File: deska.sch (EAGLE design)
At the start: 14 parts, among them T1 TIP122, T2 TIP122, T3 TIP122, X2 NAPAJENI

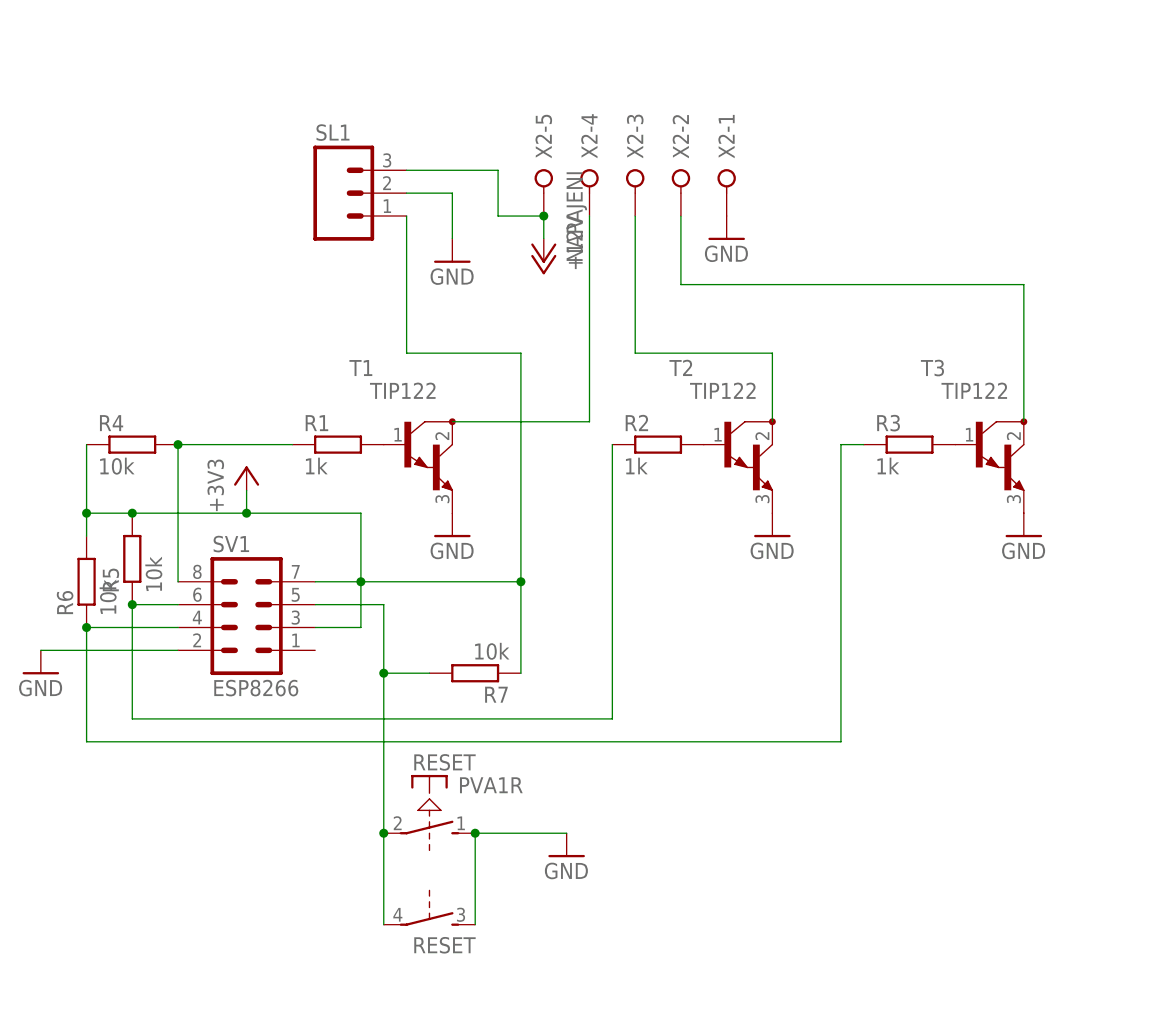
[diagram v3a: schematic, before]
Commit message: upravy desky
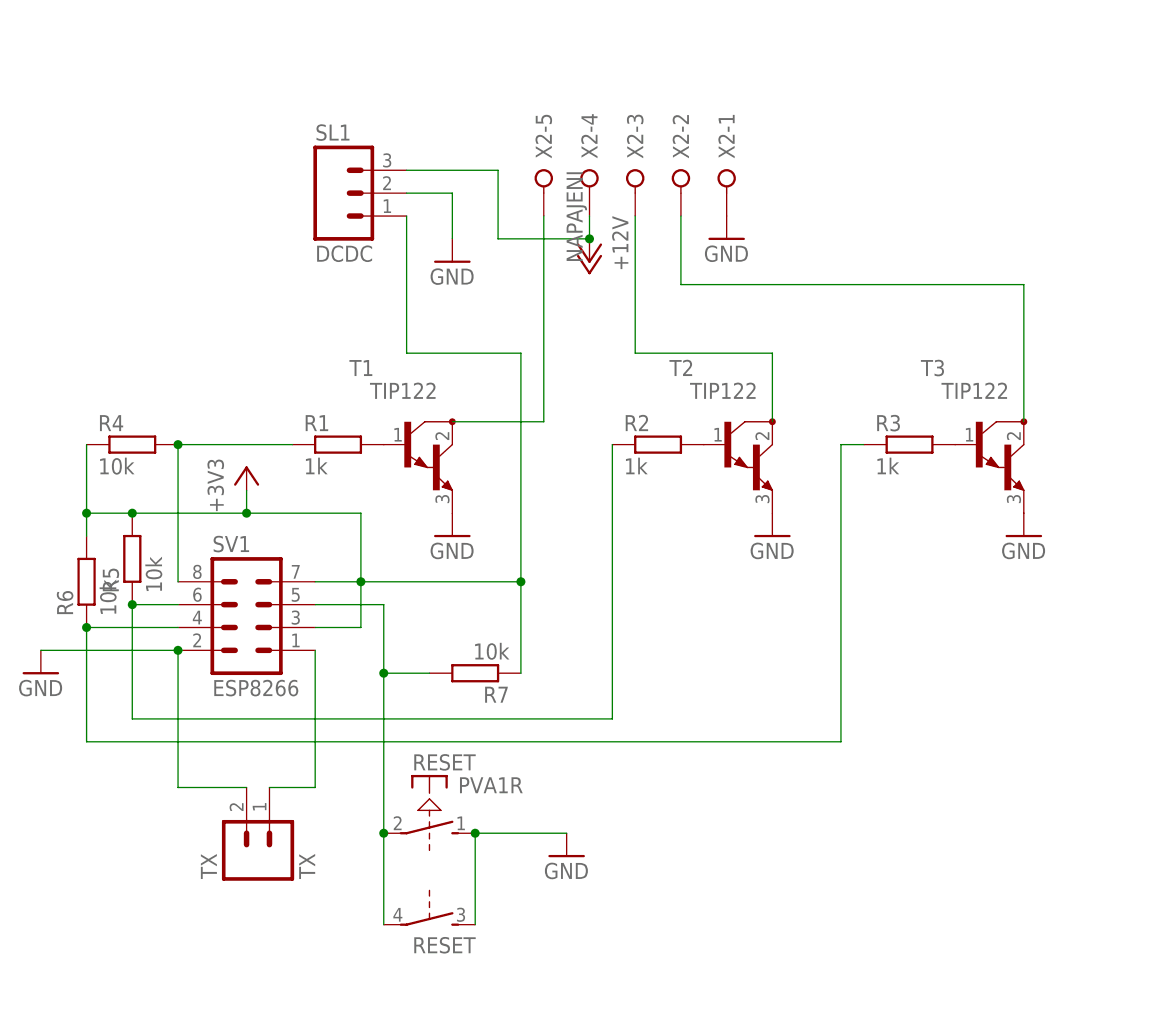
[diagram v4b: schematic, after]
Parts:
- added TX: TX, con-amp-quick:M02
- SL1: value (none) -> DCDC
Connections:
- new net N$9: SV1.1, TX.1
- net +12V: now also X2-4.KL; no longer X2-5.KL
- net GND: now also TX.2
- net N$1: now also X2-5.KL; no longer X2-4.KL
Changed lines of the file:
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@@
 <part name="GND7" library="supply1" deviceset="GND" device=""/>
 <part name="+3V1" library="supply1" library_urn="urn:adsk.eagle:library:371" deviceset="+3V3" device=""/>
-<part name="SL1" library="con-amp-quick" library_urn="urn:adsk.eagle:library:125" deviceset="M03" device="" package3d_urn="urn:adsk.eagle:package:5957/1"/>
+<part name="SL1" library="con-amp-quick" library_urn="urn:adsk.eagle:library:125" deviceset="M03" device="" package3d_urn="urn:adsk.eagle:package:5957/1" value="DCDC"/>
 <part name="GND5" library="supply1" deviceset="GND" device=""/>
+<part name="TX" library="con-amp-quick" library_urn="urn:adsk.eagle:library:125" deviceset="M02" device="" package3d_urn="urn:adsk.eagle:package:5956/1" value="TX"/>
 </parts>
 <sheets>
@@
 <instance part="GND2" gate="1" x="58.42" y="55.88"/>
 <instance part="GND3" gate="1" x="86.36" y="55.88"/>
-<instance part="P+1" gate="1" x="33.02" y="86.36" rot="R180"/>
+<instance part="P+1" gate="1" x="38.1" y="86.36" rot="R180"/>
 <instance part="R1" gate="G$1" x="10.16" y="66.04"/>
 <instance part="R2" gate="G$1" x="45.72" y="66.04"/>
@@
 <instance part="SL1" gate="G$1" x="10.16" y="93.98"/>
 <instance part="GND5" gate="1" x="22.86" y="86.36"/>
+<instance part="TX" gate="G$1" x="2.54" y="20.32" rot="R90"/>
 </instances>
 <busses>
@@
 <wire x1="-22.86" y1="43.18" x2="-7.62" y2="43.18" width="0.1524" layer="91"/>
 <pinref part="SV1" gate="G$1" pin="2"/>
+<pinref part="TX" gate="G$1" pin="2"/>
+<wire x1="0" y1="27.94" x2="-7.62" y2="27.94" width="0.1524" layer="91"/>
+<wire x1="-7.62" y1="27.94" x2="-7.62" y2="43.18" width="0.1524" layer="91"/>
+<junction x="-7.62" y="43.18"/>
 </segment>
 <segment>
@@
 </segment>
 </net>
-<net name="+12V" class="0">
-<segment>
-<pinref part="P+1" gate="1" pin="+12V"/>
-<wire x1="33.02" y1="88.9" x2="33.02" y2="91.44" width="0.1524" layer="91"/>
+<net name="N$1" class="0">
+<segment>
+<pinref part="T1" gate="G$1" pin="C"/>
+<wire x1="22.86" y1="68.58" x2="33.02" y2="68.58" width="0.1524" layer="91"/>
 <pinref part="X2" gate="-5" pin="KL"/>
-<pinref part="SL1" gate="G$1" pin="3"/>
-<wire x1="17.78" y1="96.52" x2="27.94" y2="96.52" width="0.1524" layer="91"/>
-<wire x1="27.94" y1="96.52" x2="27.94" y2="91.44" width="0.1524" layer="91"/>
-<wire x1="27.94" y1="91.44" x2="33.02" y2="91.44" width="0.1524" layer="91"/>
-<junction x="33.02" y="91.44"/>
-</segment>
-</net>
-<net name="N$1" class="0">
-<segment>
-<pinref part="T1" gate="G$1" pin="C"/>
-<wire x1="22.86" y1="68.58" x2="38.1" y2="68.58" width="0.1524" layer="91"/>
-<wire x1="38.1" y1="68.58" x2="38.1" y2="91.44" width="0.1524" layer="91"/>
-<pinref part="X2" gate="-4" pin="KL"/>
+<wire x1="33.02" y1="91.44" x2="33.02" y2="68.58" width="0.1524" layer="91"/>
 </segment>
 </net>
@@
 </segment>
 </net>
+<net name="N$9" class="0">
+<segment>
+<pinref part="SV1" gate="G$1" pin="1"/>
+<wire x1="7.62" y1="43.18" x2="7.62" y2="27.94" width="0.1524" layer="91"/>
+<pinref part="TX" gate="G$1" pin="1"/>
+<wire x1="7.62" y1="27.94" x2="2.54" y2="27.94" width="0.1524" layer="91"/>
+</segment>
+</net>
+<net name="+12V" class="0">
+<segment>
+<pinref part="X2" gate="-4" pin="KL"/>
+<pinref part="P+1" gate="1" pin="+12V"/>
+<wire x1="38.1" y1="88.9" x2="38.1" y2="91.44" width="0.1524" layer="91"/>
+<pinref part="SL1" gate="G$1" pin="3"/>
+<wire x1="17.78" y1="96.52" x2="27.94" y2="96.52" width="0.1524" layer="91"/>
+<wire x1="27.94" y1="96.52" x2="27.94" y2="88.9" width="0.1524" layer="91"/>
+<wire x1="27.94" y1="88.9" x2="38.1" y2="88.9" width="0.1524" layer="91"/>
+<junction x="38.1" y="88.9"/>
+</segment>
+</net>

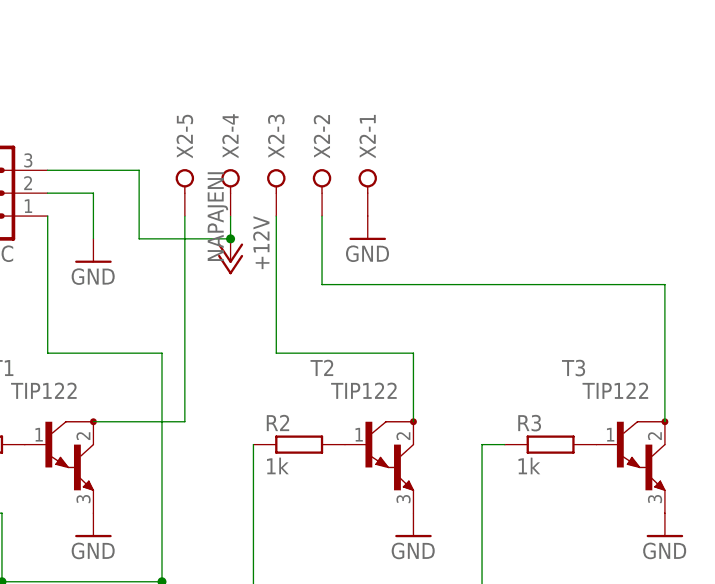
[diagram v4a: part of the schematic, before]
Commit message: deska
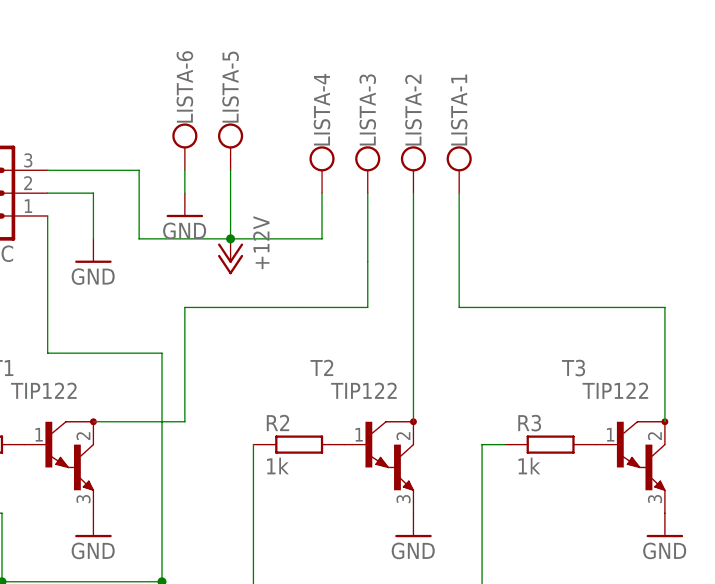
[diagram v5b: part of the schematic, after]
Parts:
- removed X2: NAPAJENI, con-wago-508:W237-05P
- added LISTA: (no value), con-wago-500:W237-6
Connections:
- net +12V: now also LISTA-4.KL, LISTA-5.KL; no longer X2-4.KL
- net GND: now also LISTA-6.KL; no longer X2-1.KL
- net N$1: now also LISTA-3.KL; no longer X2-5.KL
- net N$2: now also LISTA-2.KL; no longer X2-3.KL
- net N$3: now also LISTA-1.KL; no longer X2-2.KL
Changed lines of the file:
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@@
 <grid distance="0.1" unitdist="inch" unit="inch" style="lines" multiple="1" display="no" altdistance="0.01" altunitdist="inch" altunit="inch"/>
 <layers>
-<layer number="1" name="Top" color="4" fill="1" visible="no" active="no"/>
-<layer number="16" name="Bottom" color="1" fill="1" visible="no" active="no"/>
-<layer number="17" name="Pads" color="2" fill="1" visible="no" active="no"/>
-<layer number="18" name="Vias" color="2" fill="1" visible="no" active="no"/>
-<layer number="19" name="Unrouted" color="6" fill="1" visible="no" active="no"/>
-<layer number="20" name="Dimension" color="15" fill="1" visible="no" active="no"/>
-<layer number="21" name="tPlace" color="7" fill="1" visible="no" active="no"/>
-<layer number="22" name="bPlace" color="7" fill="1" visible="no" active="no"/>
-<layer number="23" name="tOrigins" color="15" fill="1" visible="no" active="no"/>
-<layer number="24" name="bOrigins" color="15" fill="1" visible="no" active="no"/>
-<layer number="25" name="tNames" color="7" fill="1" visible="no" active="no"/>
-<layer number="26" name="bNames" color="7" fill="1" visible="no" active="no"/>
-<layer number="27" name="tValues" color="7" fill="1" visible="no" active="no"/>
-<layer number="28" name="bValues" color="7" fill="1" visible="no" active="no"/>
+<layer number="1" name="Top" color="4" fill="1" visible="yes" active="no"/>
+<layer number="16" name="Bottom" color="1" fill="1" visible="yes" active="no"/>
+<layer number="17" name="Pads" color="2" fill="1" visible="yes" active="no"/>
+<layer number="18" name="Vias" color="2" fill="1" visible="yes" active="no"/>
+<layer number="19" name="Unrouted" color="6" fill="1" visible="yes" active="no"/>
+<layer number="20" name="Dimension" color="15" fill="1" visible="yes" active="no"/>
+<layer number="21" name="tPlace" color="7" fill="1" visible="yes" active="no"/>
+<layer number="22" name="bPlace" color="7" fill="1" visible="yes" active="no"/>
+<layer number="23" name="tOrigins" color="15" fill="1" visible="yes" active="no"/>
+<layer number="24" name="bOrigins" color="15" fill="1" visible="yes" active="no"/>
+<layer number="25" name="tNames" color="7" fill="1" visible="yes" active="no"/>
+<layer number="26" name="bNames" color="7" fill="1" visible="yes" active="no"/>
+<layer number="27" name="tValues" color="7" fill="1" visible="yes" active="no"/>
+<layer number="28" name="bValues" color="7" fill="1" visible="yes" active="no"/>
 <layer number="29" name="tStop" color="7" fill="3" visible="no" active="no"/>
 <layer number="30" name="bStop" color="7" fill="6" visible="no" active="no"/>
@@
 <layer number="35" name="tGlue" color="7" fill="4" visible="no" active="no"/>
 <layer number="36" name="bGlue" color="7" fill="5" visible="no" active="no"/>
-<layer number="37" name="tTest" color="7" fill="1" visible="no" active="no"/>
-<layer number="38" name="bTest" color="7" fill="1" visible="no" active="no"/>
+<layer number="37" name="tTest" color="7" fill="1" visible="yes" active="no"/>
+<layer number="38" name="bTest" color="7" fill="1" visible="yes" active="no"/>
 <layer number="39" name="tKeepout" color="4" fill="11" visible="no" active="no"/>
 <layer number="40" name="bKeepout" color="1" fill="11" visible="no" active="no"/>
@@
 <layer number="44" name="Drills" color="7" fill="1" visible="no" active="no"/>
 <layer number="45" name="Holes" color="7" fill="1" visible="no" active="no"/>
-<layer number="46" name="Milling" color="3" fill="1" visible="no" active="no"/>
-<layer number="47" name="Measures" color="7" fill="1" visible="no" active="no"/>
-<layer number="48" name="Document" color="7" fill="1" visible="no" active="no"/>
-<layer number="49" name="Reference" color="7" fill="1" visible="no" active="no"/>
-<layer number="51" name="tDocu" color="7" fill="1" visible="no" active="no"/>
-<layer number="52" name="bDocu" color="7" fill="1" visible="no" active="no"/>
+<layer number="46" name="Milling" color="3" fill="1" visible="yes" active="no"/>
+<layer number="47" name="Measures" color="7" fill="1" visible="yes" active="no"/>
+<layer number="48" name="Document" color="7" fill="1" visible="yes" active="no"/>
+<layer number="49" name="Reference" color="7" fill="1" visible="yes" active="no"/>
+<layer number="51" name="tDocu" color="7" fill="1" visible="yes" active="no"/>
+<layer number="52" name="bDocu" color="7" fill="1" visible="yes" active="no"/>
 <layer number="90" name="Modules" color="5" fill="1" visible="yes" active="yes"/>
 <layer number="91" name="Nets" color="2" fill="1" visible="yes" active="yes"/>
@@
 <part name="R3" library="rcl" deviceset="R-EU_" device="0207/10" value="1k"/>
 <part name="GND6" library="supply1" deviceset="GND" device=""/>
-<part name="X2" library="con-wago-508" deviceset="W237-05P" device="" value="NAPAJENI"/>
 <part name="GND4" library="supply1" deviceset="GND" device=""/>
 <part name="SV1" library="con-lstb" deviceset="MA04-2" device="" value="ESP8266"/>
@@
 <part name="GND5" library="supply1" deviceset="GND" device=""/>
 <part name="TX" library="con-amp-quick" library_urn="urn:adsk.eagle:library:125" deviceset="M02" device="" package3d_urn="urn:adsk.eagle:package:5956/1" value="TX"/>
+<part name="LISTA" library="con-wago-500" library_urn="urn:adsk.eagle:library:195" deviceset="W237-6" device="" package3d_urn="urn:adsk.eagle:package:10696/1"/>
 </parts>
 <sheets>
@@
 <instance part="R3" gate="G$1" x="73.66" y="66.04"/>
 <instance part="GND6" gate="1" x="-22.86" y="40.64"/>
-<instance part="X2" gate="-1" x="53.34" y="96.52" rot="R270"/>
-<instance part="X2" gate="-2" x="48.26" y="96.52" rot="R270"/>
-<instance part="X2" gate="-3" x="43.18" y="96.52" rot="R270"/>
-<instance part="X2" gate="-4" x="38.1" y="96.52" rot="R270"/>
-<instance part="X2" gate="-5" x="33.02" y="96.52" rot="R270"/>
-<instance part="GND4" gate="1" x="53.34" y="88.9"/>
+<instance part="GND4" gate="1" x="33.02" y="91.44"/>
 <instance part="SV1" gate="G$1" x="0" y="48.26"/>
 <instance part="R4" gate="G$1" x="-12.7" y="66.04"/>
@@
 <instance part="GND5" gate="1" x="22.86" y="86.36"/>
 <instance part="TX" gate="G$1" x="2.54" y="20.32" rot="R90"/>
+<instance part="LISTA" gate="-1" x="63.5" y="99.06" rot="R270"/>
+<instance part="LISTA" gate="-2" x="58.42" y="99.06" rot="R270"/>
+<instance part="LISTA" gate="-3" x="53.34" y="99.06" rot="R270"/>
+<instance part="LISTA" gate="-4" x="48.26" y="99.06" rot="R270"/>
+<instance part="LISTA" gate="-5" x="38.1" y="101.6" rot="R270"/>
+<instance part="LISTA" gate="-6" x="33.02" y="101.6" rot="R270"/>
 </instances>
 <busses>
@@
 </segment>
 <segment>
-<pinref part="X2" gate="-1" pin="KL"/>
-<pinref part="GND4" gate="1" pin="GND"/>
-</segment>
-<segment>
 <pinref part="RESET" gate="1" pin="S"/>
 <pinref part="RESET" gate="2" pin="S"/>
@@
 <wire x1="22.86" y1="93.98" x2="22.86" y2="88.9" width="0.1524" layer="91"/>
 </segment>
+<segment>
+<pinref part="LISTA" gate="-6" pin="KL"/>
+<pinref part="GND4" gate="1" pin="GND"/>
+<wire x1="33.02" y1="93.98" x2="33.02" y2="96.52" width="0.1524" layer="91"/>
+</segment>
 </net>
 <net name="N$1" class="0">
@@
 <pinref part="T1" gate="G$1" pin="C"/>
 <wire x1="22.86" y1="68.58" x2="33.02" y2="68.58" width="0.1524" layer="91"/>
-<pinref part="X2" gate="-5" pin="KL"/>
-<wire x1="33.02" y1="91.44" x2="33.02" y2="68.58" width="0.1524" layer="91"/>
+<pinref part="LISTA" gate="-3" pin="KL"/>
+<wire x1="53.34" y1="93.98" x2="53.34" y2="86.36" width="0.1524" layer="91"/>
+<wire x1="53.34" y1="86.36" x2="53.34" y2="81.28" width="0.1524" layer="91"/>
+<wire x1="53.34" y1="81.28" x2="45.72" y2="81.28" width="0.1524" layer="91"/>
+<wire x1="45.72" y1="81.28" x2="33.02" y2="81.28" width="0.1524" layer="91"/>
+<wire x1="33.02" y1="81.28" x2="33.02" y2="68.58" width="0.1524" layer="91"/>
 </segment>
 </net>
 <net name="N$2" class="0">
 <segment>
-<wire x1="43.18" y1="91.44" x2="43.18" y2="76.2" width="0.1524" layer="91"/>
 <pinref part="T2" gate="G$1" pin="C"/>
-<wire x1="43.18" y1="76.2" x2="58.42" y2="76.2" width="0.1524" layer="91"/>
 <wire x1="58.42" y1="76.2" x2="58.42" y2="68.58" width="0.1524" layer="91"/>
-<pinref part="X2" gate="-3" pin="KL"/>
+<pinref part="LISTA" gate="-2" pin="KL"/>
+<wire x1="58.42" y1="93.98" x2="58.42" y2="76.2" width="0.1524" layer="91"/>
 </segment>
 </net>
@@
 <segment>
 <pinref part="T3" gate="G$1" pin="C"/>
-<wire x1="48.26" y1="91.44" x2="48.26" y2="83.82" width="0.1524" layer="91"/>
-<wire x1="48.26" y1="83.82" x2="86.36" y2="83.82" width="0.1524" layer="91"/>
-<wire x1="86.36" y1="83.82" x2="86.36" y2="68.58" width="0.1524" layer="91"/>
-<pinref part="X2" gate="-2" pin="KL"/>
+<pinref part="LISTA" gate="-1" pin="KL"/>
+<wire x1="86.36" y1="81.28" x2="86.36" y2="68.58" width="0.1524" layer="91"/>
+<wire x1="63.5" y1="93.98" x2="63.5" y2="81.28" width="0.1524" layer="91"/>
+<wire x1="63.5" y1="81.28" x2="86.36" y2="81.28" width="0.1524" layer="91"/>
 </segment>
 </net>
@@
 <net name="+12V" class="0">
 <segment>
-<pinref part="X2" gate="-4" pin="KL"/>
 <pinref part="P+1" gate="1" pin="+12V"/>
-<wire x1="38.1" y1="88.9" x2="38.1" y2="91.44" width="0.1524" layer="91"/>
 <pinref part="SL1" gate="G$1" pin="3"/>
 <wire x1="17.78" y1="96.52" x2="27.94" y2="96.52" width="0.1524" layer="91"/>
 <wire x1="27.94" y1="96.52" x2="27.94" y2="88.9" width="0.1524" layer="91"/>
 <wire x1="27.94" y1="88.9" x2="38.1" y2="88.9" width="0.1524" layer="91"/>
+<pinref part="LISTA" gate="-5" pin="KL"/>
+<wire x1="38.1" y1="96.52" x2="38.1" y2="88.9" width="0.1524" layer="91"/>
 <junction x="38.1" y="88.9"/>
-</segment>
-</net>
+<wire x1="38.1" y1="88.9" x2="48.26" y2="88.9" width="0.1524" layer="91"/>
+<pinref part="LISTA" gate="-4" pin="KL"/>
+<wire x1="48.26" y1="88.9" x2="48.26" y2="93.98" width="0.1524" layer="91"/>
+</segment>
+</net>
